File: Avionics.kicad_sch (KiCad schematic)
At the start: 40 parts, among them Q21 IRLML2803, SW1 KMR231NG LFS, U1 MAX706RESA+, U2 ATSAMD51J20A-AU, U3 BMX160, U4 DS3231S, U5 MR25H40MDF, Y1 32.768kHz

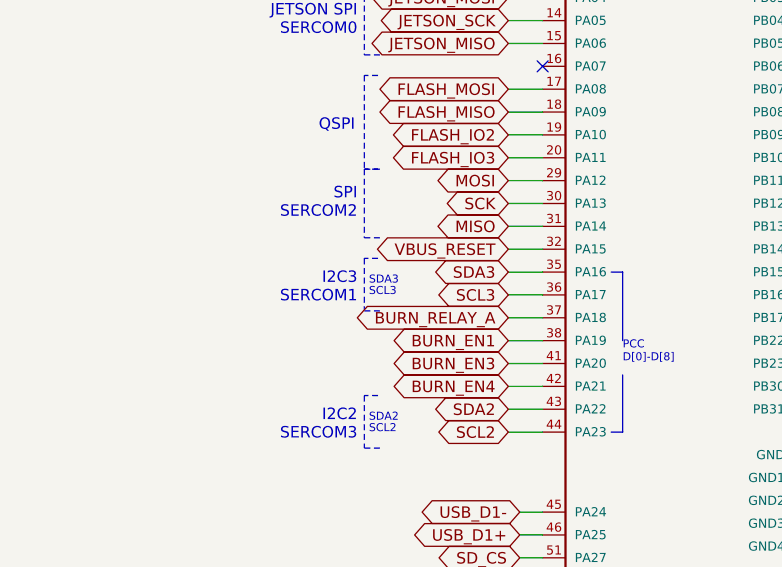
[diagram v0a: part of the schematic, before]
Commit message: Stash
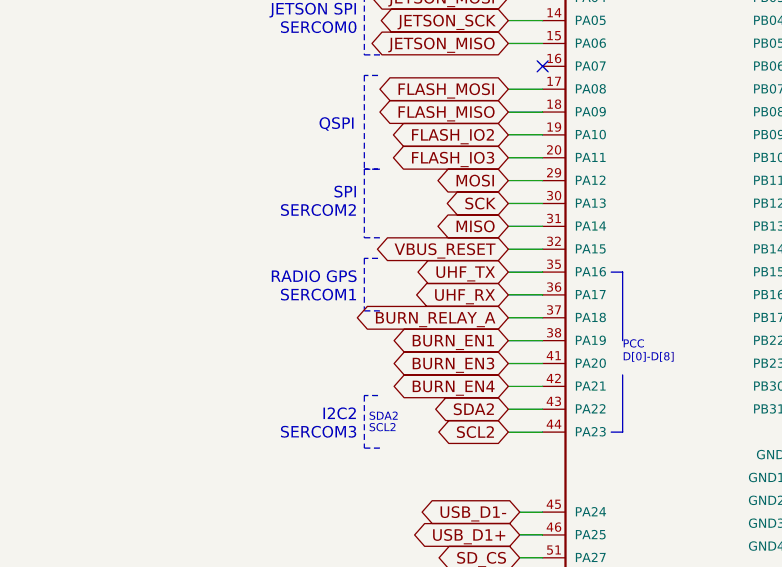
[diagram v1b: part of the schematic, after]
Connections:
- net SCL3 renamed UHF_RX
- net SDA3 renamed UHF_TX
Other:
- note added: "RADIO GPS SERCOM1"
- note removed: "I2C3 SERCOM1"
- note removed: "SCL3"
- note removed: "SDA3"
